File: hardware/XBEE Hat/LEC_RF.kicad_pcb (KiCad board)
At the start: 2 copper layers, 70 x 40 mm, 6 parts, among them J1 Conn_Coaxial_Small, J2 Conn_01x04, U1 XBee_SMT, U2 TLV1117-33

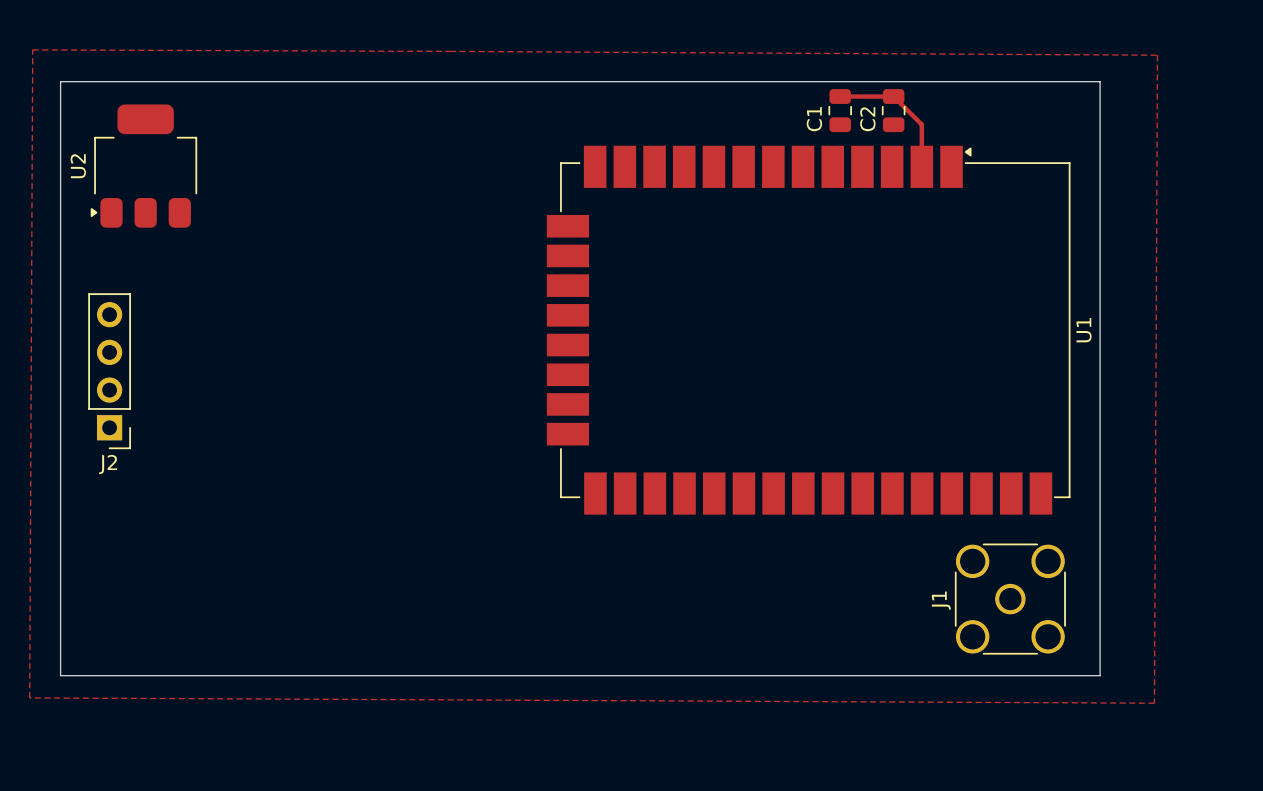
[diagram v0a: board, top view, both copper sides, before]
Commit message: Push of most recent schematic and PCB
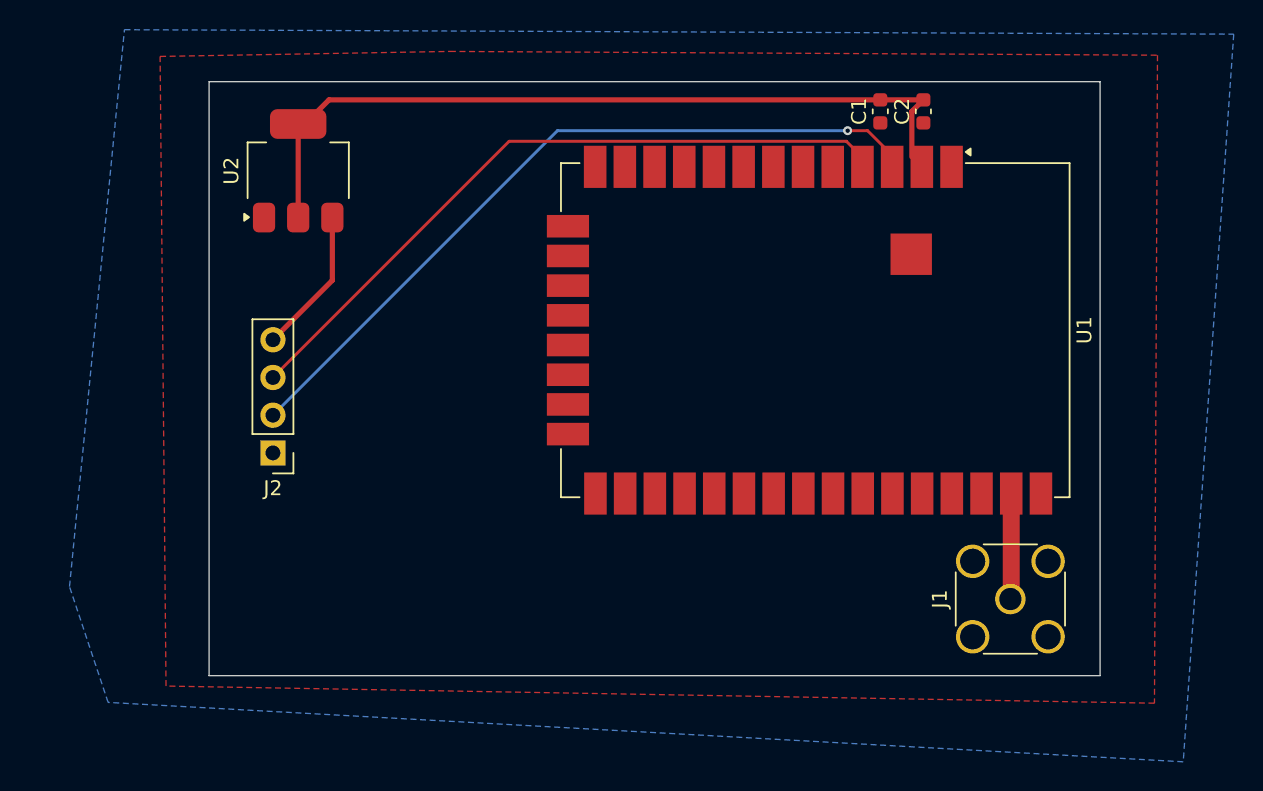
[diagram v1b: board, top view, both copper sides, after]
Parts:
- C1, C2: footprint Capacitor_SMD:C_0805_2012Metric -> Capacitor_SMD:C_0603_1608Metric
- U1: footprint RF_Module:Digi_XBee_SMT -> Custom:XBEE_GND_PAD
- moved J2 11.1 mm to (84.3, 85.0)
- moved U2 10.3 mm to (86.0, 66.0)
- moved C1 2.70 mm to (125.2, 62.0)
- moved C2 2.00 mm to (128.1, 62.0)
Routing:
- net UART_TX: track 0.00 -> 51.1 mm, vias 0 -> 1
- net UART_RX: track 0.00 -> 47.4 mm
- net +3.3V: track 9.13 -> 54.2 mm
- net +5V: track 0.00 -> 9.89 mm
- net Net-(J1-In): track 0.00 -> 7.13 mm
- added copper zone on B.Cu, net GND
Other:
- board size 70 x 40 mm -> 60 x 40 mm
